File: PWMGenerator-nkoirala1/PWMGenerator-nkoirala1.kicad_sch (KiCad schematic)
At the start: 7 parts, among them J1 Barrel_Jack, J2 Conn_01x03_Pin, Q1 NPN, Q2 PNP, U1 LM7805_TO220

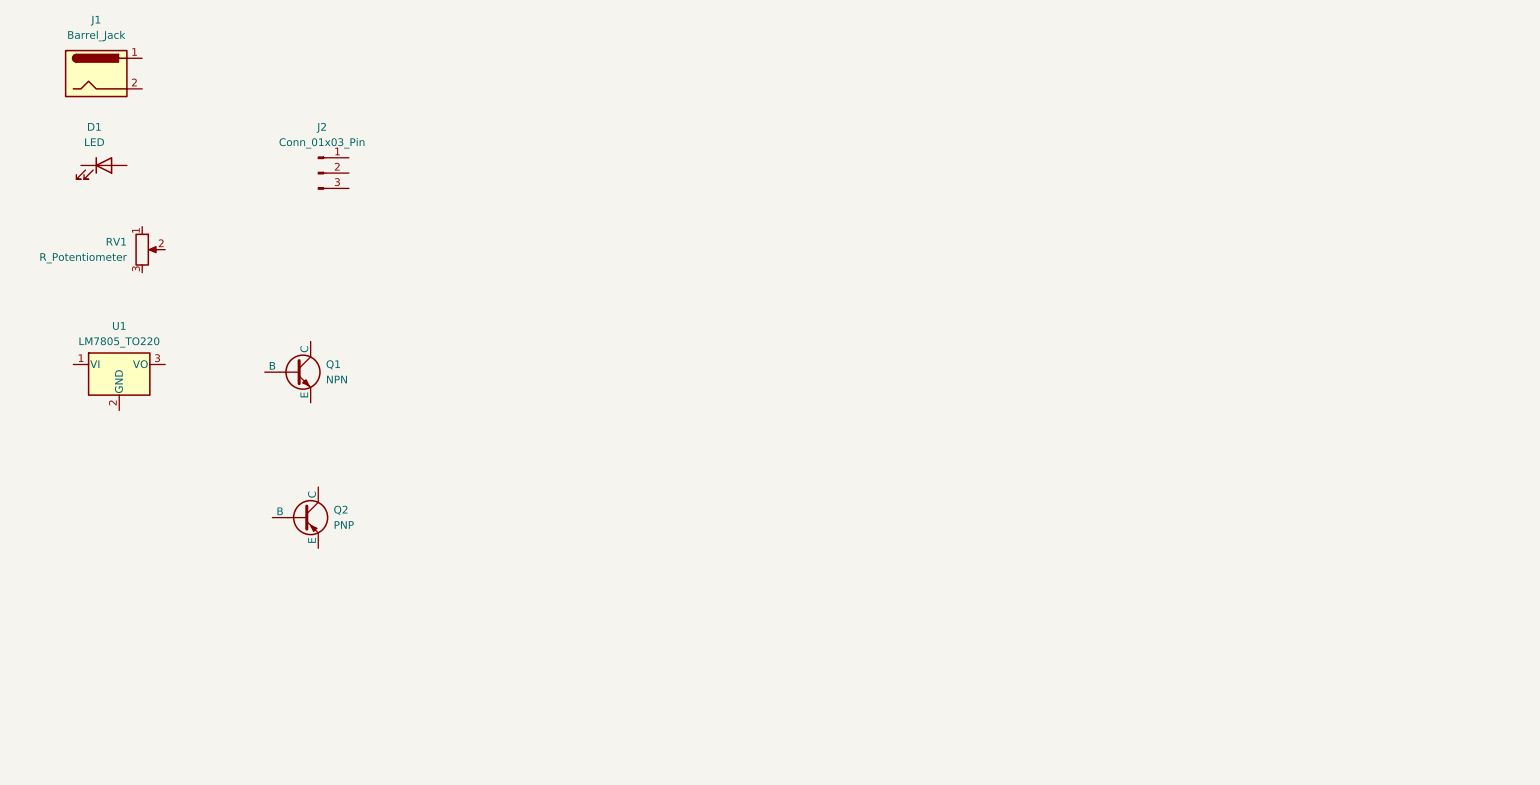
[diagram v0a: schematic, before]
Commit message: placed all the components
done
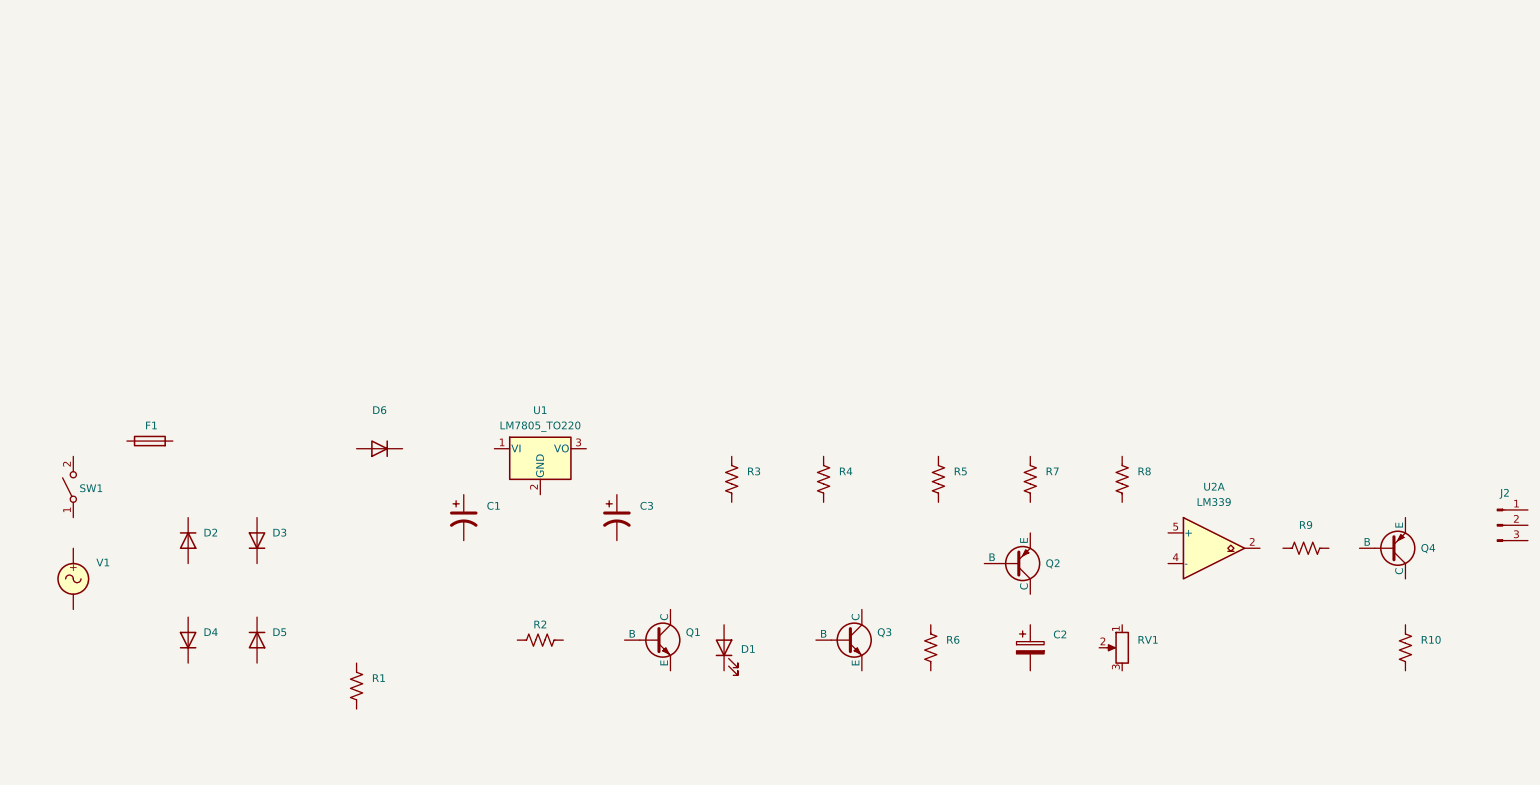
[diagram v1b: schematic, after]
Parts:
- removed J1: Barrel_Jack, Connector_BarrelJack:BarrelJack_CLIFF_FC681465S_SMT_Horizontal, symbol Connector:Barrel_Jack
- added C1, C3: C_Polarized_US, symbol Device:C_Polarized_US
- added C2: C_Polarized, symbol Device:C_Polarized
- added D2, D3, D4, D5, D6: 1N4005, Diode_THT:D_DO-41_SOD81_P10.16mm_Horizontal, symbol Diode:1N4005
- added F1: Fuse, symbol Device:Fuse
- added Q3: NPN, Package_TO_SOT_THT:TO-92, symbol Simulation_SPICE:NPN
- added Q4: PNP, Package_TO_SOT_THT:TO-92, symbol Simulation_SPICE:PNP
- added R1, R10, R2, R3, R4, R5, R6, R7, R8, R9: R_US, symbol Device:R_US
- added SW1: SW_SPST, symbol Switch:SW_SPST
- added U2: LM339, symbol Comparator:LM339
- added V1: VSIN, symbol Simulation_SPICE:VSIN
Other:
- moved on the sheet: D1, J2, Q1, Q2, RV1, U1

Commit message: commit wiring done
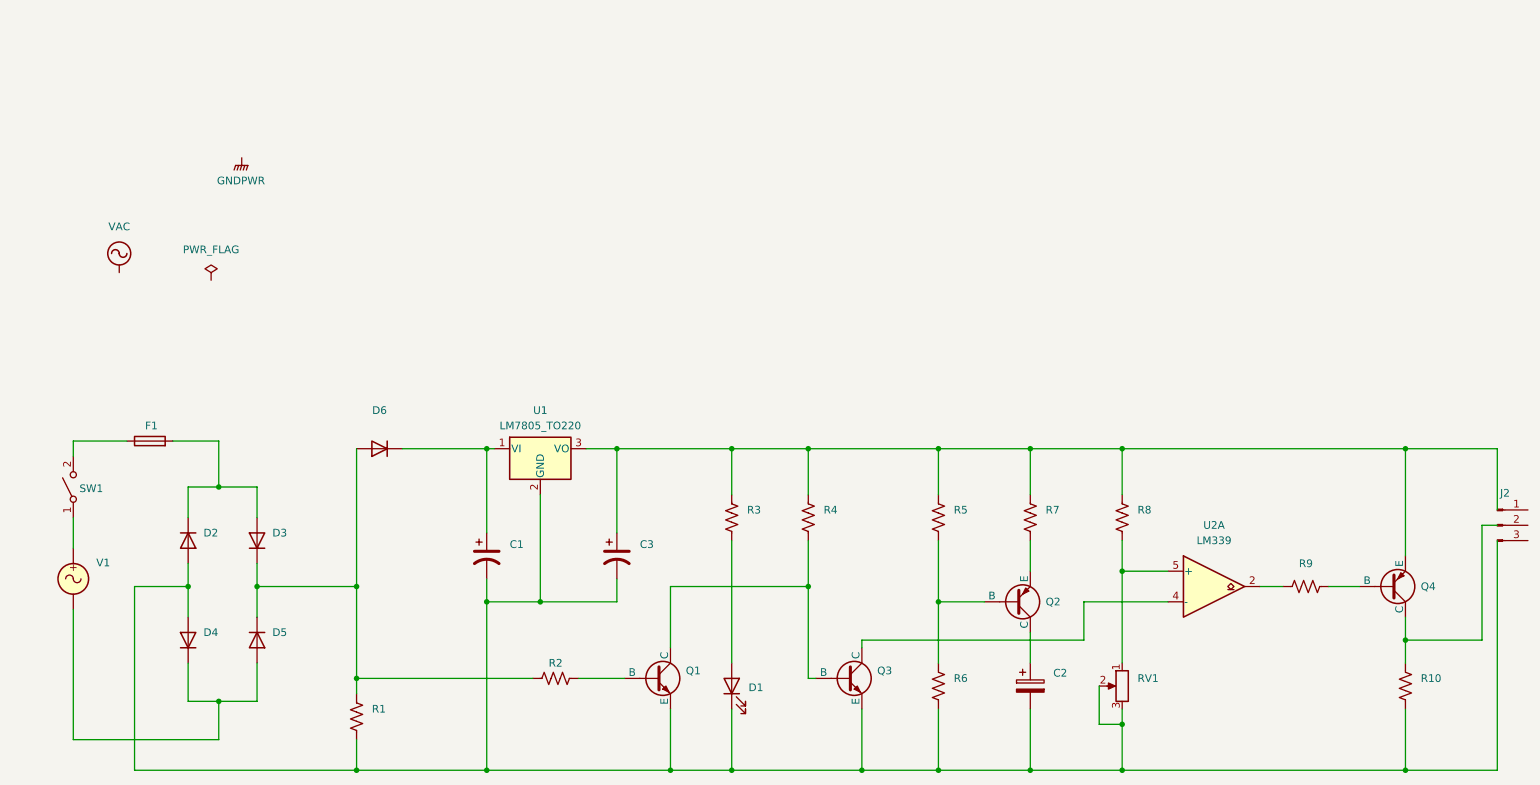
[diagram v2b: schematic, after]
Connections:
- net at D5.1 (K): now also D3.1 (K), D6.2 (A), R1.1, R2.1
- net at D5.2 (A): now also D4.1 (K), V1.2
- net at R5.1: now also C3.1, Q4.3 (E), R3.1, R4.1, R7.1, R8.1, U1.3 (VO)
- net at R5.2: now also Q2.2 (B), R6.1
- net at R3.2: now also D1.2 (A)
- net at U1.1 (VI): now also C1.1, D6.1 (K)
- net at U1.2 (GND): now also C1.2, C2.2, C3.2, D1.1 (K), D2.2 (A), D4.2 (A), Q1.3 (E), Q3.3 (E), R1.2, R10.2, R6.2, RV1.2, RV1.3
- net at SW1.1 (A): now also V1.1
- net at SW1.2 (B): now also F1.1
- net at RV1.1: now also R8.2, U2.5 (+)
- net at D2.1 (K): now also D3.2 (A), F1.2
- net at Q3.1 (C): now also U2.4 (-)
- net at Q3.2 (B): now also Q1.1 (C), R4.2
- net at R7.2: now also Q2.3 (E)
- net at R2.2: now also Q1.2 (B)
- net at Q2.1 (C): now also C2.1
- net at R9.1: now also U2.2
- net at R9.2: now also Q4.2 (B)
- net at Q4.1 (C): now also R10.1
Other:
- moved on the sheet: C1, C2, C3, D1, Q1, Q2, Q3, Q4, R1, R10, R2, R3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
